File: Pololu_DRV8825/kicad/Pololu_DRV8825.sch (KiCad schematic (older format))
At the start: 24 parts, among them J1 CONN_01X02, J2 CONN_01X02, J3 CONN_01X02, P1 CONN_01X10, P2 CONN_01X10, P3 CONN_02X10, P4 CONN_02X10, P5 CONN_01X04, P6 CONN_01X04, U1 MSP430G2553IN20, U2 LM2931Z-3.3/5.0, U3 Pololu_DRV8825, U4 Pololu_DRV8825

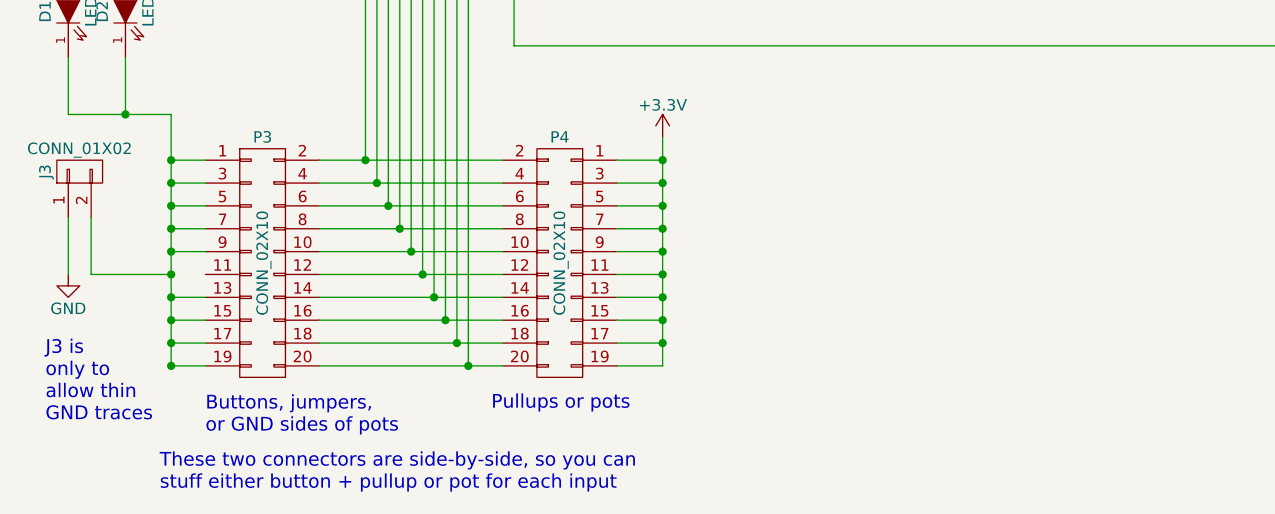
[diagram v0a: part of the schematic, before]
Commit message: Ready for first manufacturing run
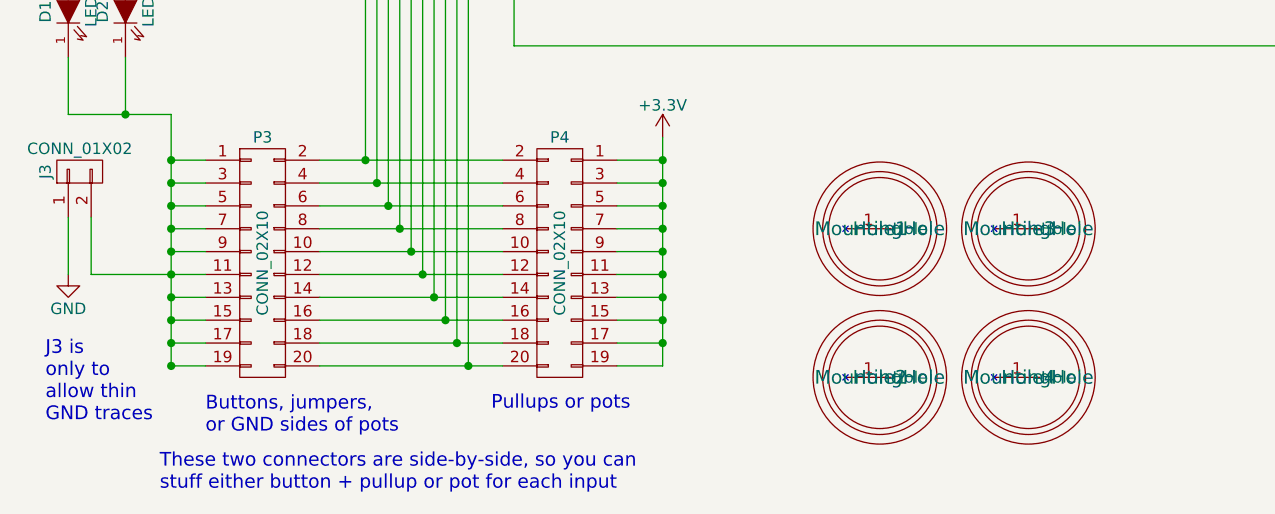
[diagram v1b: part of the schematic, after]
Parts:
- added Hole1, Hole2, Hole3, Hole4: MountingHole, Connect:1pin, symbol MountingHole
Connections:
- net at D1.1 (K), D2.1 (K), J3.2 (P2)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: now also P3.11 (P11)
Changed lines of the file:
@@
 $EndComp
 $Comp
-L GND #PWR025
+L GND #PWR023
 U 1 1 55E92FCD
 P 5100 2550
-F 0 "#PWR025" H 5100 2300 50  0001 C CNN
+F 0 "#PWR023" H 5100 2300 50  0001 C CNN
 F 1 "GND" H 5100 2400 50  0000 C CNN
 F 2 "" H 5100 2550 60  0000 C CNN
@@
 $EndComp
 $Comp
-L +3.3V #PWR026
+L +3.3V #PWR024
 U 1 1 55EA1205
 P 3300 6150
-F 0 "#PWR026" H 3300 6000 50  0001 C CNN
+F 0 "#PWR024" H 3300 6000 50  0001 C CNN
 F 1 "+3.3V" H 3300 6290 50  0000 C CNN
 F 2 "" H 3300 6150 60  0000 C CNN
@@
 Connection ~ 1150 6650
 Wire Wire Line
-	800  6750 1150 6750
+	800  6750 1300 6750
 Connection ~ 1150 6750
 Wire Wire Line
@@
 	800  6500 800  6750
 $Comp
-L GND #PWR027
+L GND #PWR025
 U 1 1 55E9E96F
 P 700 6750
-F 0 "#PWR027" H 700 6500 50  0001 C CNN
+F 0 "#PWR025" H 700 6500 50  0001 C CNN
 F 1 "GND" H 700 6600 50  0000 C CNN
 F 2 "" H 700 6750 60  0000 C CNN
@@
 Connection ~ 1150 6250
 Connection ~ 950  6050
+$Comp
+L MountingHole Hole1
+U 1 1 55E9FF79
+P 4250 6550
+F 0 "Hole1" H 4250 6550 60  0000 C CNN
+F 1 "MountingHole" H 4250 6550 60  0000 C CNN
+F 2 "Connect:1pin" H 4250 6550 60  0001 C CNN
+F 3 "" H 4250 6550 60  0000 C CNN
+	1    4250 6550
+	1    0    0    -1
+$EndComp
+$Comp
+L MountingHole Hole3
+U 1 1 55E9FFFF
+P 4900 6550
+F 0 "Hole3" H 4900 6550 60  0000 C CNN
+F 1 "MountingHole" H 4900 6550 60  0000 C CNN
+F 2 "Connect:1pin" H 4900 6550 60  0001 C CNN
+F 3 "" H 4900 6550 60  0000 C CNN
+	1    4900 6550
+	1    0    0    -1
+$EndComp
+$Comp
+L MountingHole Hole2
+U 1 1 55EA0073
+P 4250 7200
+F 0 "Hole2" H 4250 7200 60  0000 C CNN
+F 1 "MountingHole" H 4250 7200 60  0000 C CNN
+F 2 "Connect:1pin" H 4250 7200 60  0001 C CNN
+F 3 "" H 4250 7200 60  0000 C CNN
+	1    4250 7200
+	1    0    0    -1
+$EndComp
+$Comp
+L MountingHole Hole4
+U 1 1 55EA00FC
+P 4900 7200
+F 0 "Hole4" H 4900 7200 60  0000 C CNN
+F 1 "MountingHole" H 4900 7200 60  0000 C CNN
+F 2 "Connect:1pin" H 4900 7200 60  0001 C CNN
+F 3 "" H 4900 7200 60  0000 C CNN
+	1    4900 7200
+	1    0    0    -1
+$EndComp
 $EndSCHEMATC
